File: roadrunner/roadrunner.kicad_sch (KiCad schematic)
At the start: 48 parts, among them J1 Battery_conn, J2 battery_conn_r, SW1 SW_Push, SW10 SW_Push, SW10_r1 SW_Push, SW11 SW_Push, SW11_r1 SW_Push, SW12 SW_Push, SW12_r1 SW_Push, SW13 SW_Push, SW13_r1 SW_Push, SW14 SW_Push, SW14_r1 SW_Push, SW15 SW_Push, SW15_r1 SW_Push, SW16 SW_Push, SW16_r1 SW_Push, SW17 SW_Push, SW17_r1 SW_Push, SW1_r1 SW_Push, SW2 SW_Push, SW2_r1 SW_Push, SW3 SW_Push, SW3_r1 SW_Push, SW4 SW_Push, SW4_r1 SW_Push, SW5 SW_Push, SW5_r1 SW_Push, SW6 SW_Push, SW6_r1 SW_Push, SW7 SW_Push, SW7_r1 SW_Push, SW8 SW_Push, SW8_r1 SW_Push, SW9 SW_Push, SW9_r1 SW_Push, U1 ProMicro-kbd, U2 ProMicro-kbd

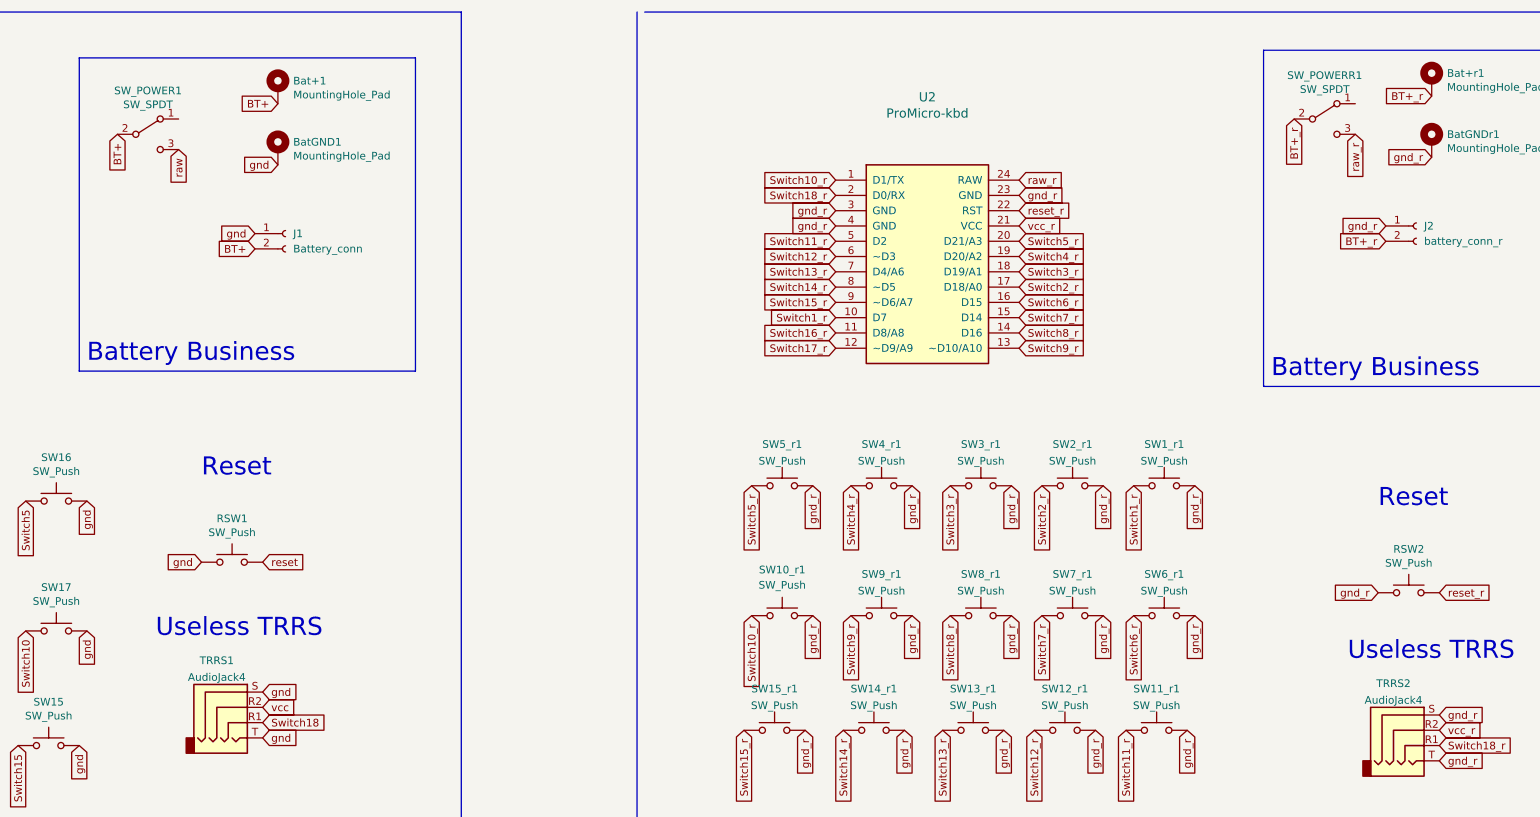
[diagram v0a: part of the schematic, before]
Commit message: update shape
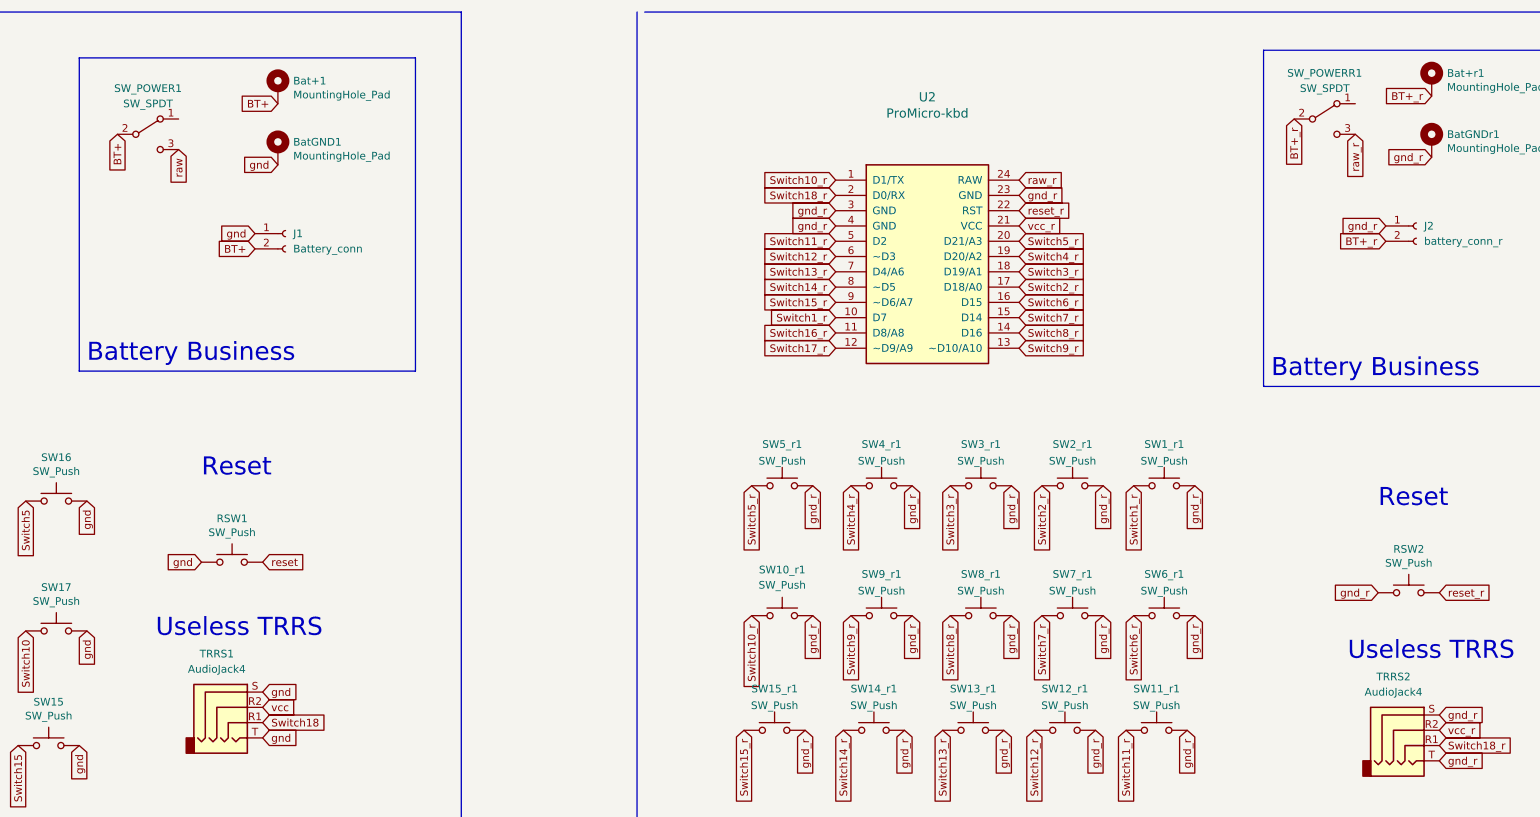
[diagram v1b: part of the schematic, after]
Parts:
- TRRS1, TRRS2: footprint (none) -> Connector_Audio:Jack_3.5mm_PJ320E_Horizontal
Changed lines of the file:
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@@
   (symbol (lib_id "Connector:AudioJack4") (at 331.47 133.35 0) (unit 1)
     (in_bom yes) (on_board yes) (fields_autoplaced)
-    (property "Reference" "TRRS2" (id 0) (at 328.93 125.5735 0))
-    (property "Value" "AudioJack4" (id 1) (at 328.93 128.3486 0))
-    (property "Footprint" "" (id 2) (at 331.47 133.35 0)
+    (property "Reference" "TRRS2" (id 0) (at 328.93 124.46 0))
+    (property "Value" "AudioJack4" (id 1) (at 328.93 127 0))
+    (property "Footprint" "Connector_Audio:Jack_3.5mm_PJ320E_Horizontal" (id 2) (at 331.47 133.35 0)
       (effects (font (size 1.27 1.27)) hide)
     )
@@
   (symbol (lib_id "Connector:AudioJack4") (at 135.89 129.54 0) (unit 1)
     (in_bom yes) (on_board yes) (fields_autoplaced)
-    (property "Reference" "TRRS1" (id 0) (at 133.35 121.7635 0))
-    (property "Value" "AudioJack4" (id 1) (at 133.35 124.5386 0))
-    (property "Footprint" "" (id 2) (at 135.89 129.54 0)
+    (property "Reference" "TRRS1" (id 0) (at 133.35 120.65 0))
+    (property "Value" "AudioJack4" (id 1) (at 133.35 123.19 0))
+    (property "Footprint" "Connector_Audio:Jack_3.5mm_PJ320E_Horizontal" (id 2) (at 135.89 129.54 0)
       (effects (font (size 1.27 1.27)) hide)
     )
@@
   )
   (symbol (lib_id "Switch:SW_SPDT") (at 121.92 34.29 0) (unit 1)
-    (in_bom yes) (on_board yes)
-    (property "Reference" "SW_POWER1" (id 0) (at 121.92 27.051 0))
-    (property "Value" "SW_SPDT" (id 1) (at 121.92 29.3624 0))
+    (in_bom yes) (on_board yes) (fields_autoplaced)
+    (property "Reference" "SW_POWER1" (id 0) (at 121.92 26.67 0))
+    (property "Value" "SW_SPDT" (id 1) (at 121.92 29.21 0))
     (property "Footprint" "battery_switch:SPDT_C128955" (id 2) (at 121.92 34.29 0)
       (effects (font (size 1.27 1.27)) hide)
@@
   )
   (symbol (lib_id "Switch:SW_SPDT") (at 317.5 31.75 0) (unit 1)
-    (in_bom yes) (on_board yes)
-    (property "Reference" "SW_POWERR1" (id 0) (at 317.5 24.511 0))
-    (property "Value" "SW_SPDT" (id 1) (at 317.5 26.8224 0))
+    (in_bom yes) (on_board yes) (fields_autoplaced)
+    (property "Reference" "SW_POWERR1" (id 0) (at 317.5 24.13 0))
+    (property "Value" "SW_SPDT" (id 1) (at 317.5 26.67 0))
     (property "Footprint" "battery_switch:SPDT_C128955" (id 2) (at 317.5 31.75 0)
       (effects (font (size 1.27 1.27)) hide)
@@
     )
     (path "/5707fb00-48c3-46d9-8f62-42ff2e9ad9f5"
-      (reference "TRRS1") (unit 1) (value "AudioJack4") (footprint "")
+      (reference "TRRS1") (unit 1) (value "AudioJack4") (footprint "Connector_Audio:Jack_3.5mm_PJ320E_Horizontal")
     )
     (path "/5340d998-a6ef-44fa-806e-718c814691ee"
-      (reference "TRRS2") (unit 1) (value "AudioJack4") (footprint "")
+      (reference "TRRS2") (unit 1) (value "AudioJack4") (footprint "Connector_Audio:Jack_3.5mm_PJ320E_Horizontal")
     )
     (path "/6801880a-11a2-4a6a-9688-e81ed1f59985"

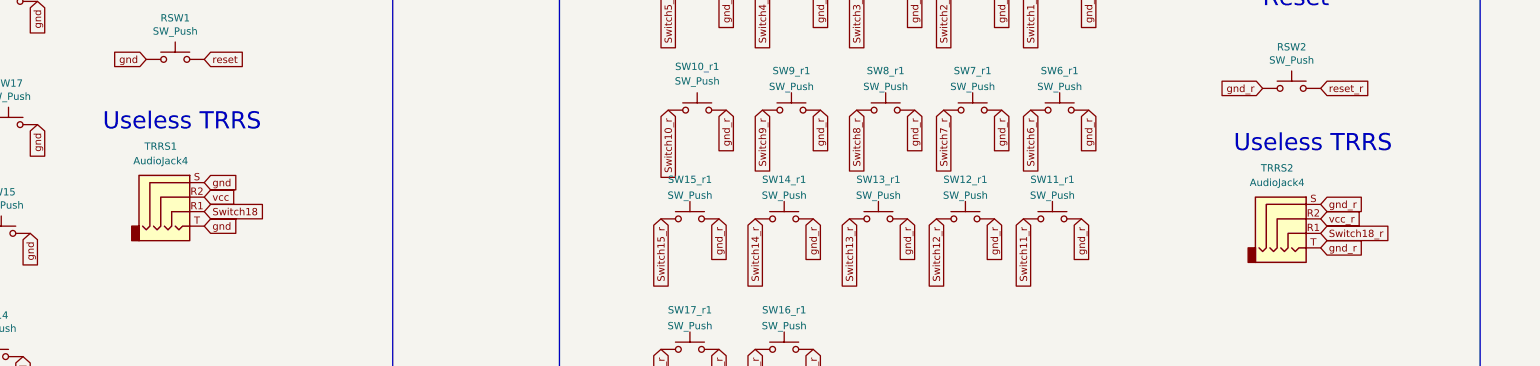
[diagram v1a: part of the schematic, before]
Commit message: basic v2 designs
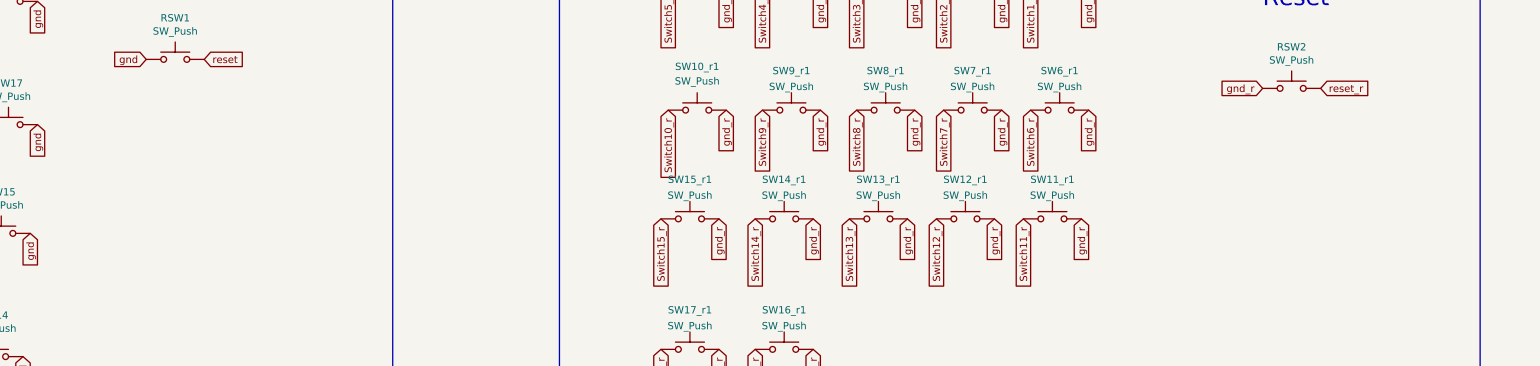
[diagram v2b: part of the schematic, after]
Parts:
- removed TRRS1, TRRS2: AudioJack4, Connector_Audio:Jack_3.5mm_PJ320E_Horizontal, symbol Connector:AudioJack4
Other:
- note removed: "Useless TRRS"
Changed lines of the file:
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@@
-    (effects (font (size 2.9972 2.9972)) (justify left bottom))
-  )
-  (text "Useless TRRS\n" (at 321.31 121.92 0)
     (effects (font (size 2.9972 2.9972)) (justify left bottom))
   )
@@
     (effects (font (size 2.9972 2.9972)) (justify left bottom))
   )
-  (text "Useless TRRS\n" (at 123.19 118.11 0)
-    (effects (font (size 2.9972 2.9972)) (justify left bottom))
-  )
   (text "Battery Business" (at 308.61 74.93 0)
     (effects (font (size 2.9972 2.9972)) (justify left bottom))
@@
     )
   )
-  (global_label "vcc_r" (shape input) (at 336.55 133.35 0) (fields_autoplaced)
-    (effects (font (size 1.27 1.27)) (justify left))
-    (property "Intersheet References" "${INTERSHEET_REFS}" (id 0) (at 343.7728 133.2706 0)
-      (effects (font (size 1.27 1.27)) (justify left) hide)
-    )
-  )
   (global_label "gnd" (shape input) (at 80.01 95.25 270) (fields_autoplaced)
     (effects (font (size 1.27 1.27)) (justify right))
     (property "Intersheet References" "${INTERSHEET_REFS}" (id 0) (at 13.97 66.04 0)
-      (effects (font (size 1.27 1.27)) hide)
-    )
-  )
-  (global_label "gnd" (shape input) (at 140.97 134.62 0) (fields_autoplaced)
-    (effects (font (size 1.27 1.27)) (justify left))
-    (property "Intersheet References" "${INTERSHEET_REFS}" (id 0) (at 13.97 67.31 0)
       (effects (font (size 1.27 1.27)) hide)
     )
@@
     )
   )
-  (global_label "gnd" (shape input) (at 140.97 127 0) (fields_autoplaced)
-    (effects (font (size 1.27 1.27)) (justify left))
-    (property "Intersheet References" "${INTERSHEET_REFS}" (id 0) (at 13.97 59.69 0)
-      (effects (font (size 1.27 1.27)) hide)
-    )
-  )
   (global_label "Switch5" (shape input) (at 101.6 95.25 270) (fields_autoplaced)
     (effects (font (size 1.27 1.27)) (justify right))
@@
     (property "Intersheet References" "${INTERSHEET_REFS}" (id 0) (at 13.97 66.04 0)
       (effects (font (size 1.27 1.27)) hide)
-    )
-  )
-  (global_label "gnd_r" (shape input) (at 336.55 130.81 0) (fields_autoplaced)
-    (effects (font (size 1.27 1.27)) (justify left))
-    (property "Intersheet References" "${INTERSHEET_REFS}" (id 0) (at 344.0752 130.8894 0)
-      (effects (font (size 1.27 1.27)) (justify left) hide)
     )
   )
@@
     )
   )
-  (global_label "gnd_r" (shape input) (at 336.55 138.43 0) (fields_autoplaced)
-    (effects (font (size 1.27 1.27)) (justify left))
-    (property "Intersheet References" "${INTERSHEET_REFS}" (id 0) (at 344.0752 138.5094 0)
-      (effects (font (size 1.27 1.27)) (justify left) hide)
-    )
-  )
   (global_label "raw" (shape input) (at 127 36.83 270) (fields_autoplaced)
     (effects (font (size 1.27 1.27)) (justify right))
@@
     )
   )
-  (global_label "Switch18" (shape input) (at 140.97 132.08 0) (fields_autoplaced)
-    (effects (font (size 1.27 1.27)) (justify left))
-    (property "Intersheet References" "${INTERSHEET_REFS}" (id 0) (at 13.97 67.31 0)
-      (effects (font (size 1.27 1.27)) hide)
-    )
-  )
   (global_label "reset_r" (shape input) (at 336.55 110.49 0) (fields_autoplaced)
     (effects (font (size 1.27 1.27)) (justify left))
@@
     )
   )
-  (global_label "vcc" (shape input) (at 140.97 129.54 0) (fields_autoplaced)
-    (effects (font (size 1.27 1.27)) (justify left))
-    (property "Intersheet References" "${INTERSHEET_REFS}" (id 0) (at 13.97 59.69 0)
-      (effects (font (size 1.27 1.27)) hide)
-    )
-  )
   (global_label "gnd_r" (shape input) (at 265.43 92.71 270) (fields_autoplaced)
     (effects (font (size 1.27 1.27)) (justify right))
@@
     (property "Intersheet References" "${INTERSHEET_REFS}" (id 0) (at 285.6706 104.1056 90)
       (effects (font (size 1.27 1.27)) (justify right) hide)
-    )
-  )
-  (global_label "Switch18_r" (shape input) (at 336.55 135.89 0) (fields_autoplaced)
-    (effects (font (size 1.27 1.27)) (justify left))
-    (property "Intersheet References" "${INTERSHEET_REFS}" (id 0) (at 208.28 -27.94 0)
-      (effects (font (size 1.27 1.27)) hide)
     )
   )
@@
     (pin "2")
   )
-  (symbol (lib_id "Connector:AudioJack4") (at 331.47 133.35 0) (unit 1)
-    (in_bom yes) (on_board yes) (fields_autoplaced)
-    (property "Reference" "TRRS2" (id 0) (at 328.93 124.46 0))
-    (property "Value" "AudioJack4" (id 1) (at 328.93 127 0))
-    (property "Footprint" "Connector_Audio:Jack_3.5mm_PJ320E_Horizontal" (id 2) (at 331.47 133.35 0)
-      (effects (font (size 1.27 1.27)) hide)
-    )
-    (property "Datasheet" "~" (id 3) (at 331.47 133.35 0)
-      (effects (font (size 1.27 1.27)) hide)
-    )
-    (pin "R1")
-    (pin "R2")
-    (pin "S")
-    (pin "T")
-  )
-  (symbol (lib_id "Connector:AudioJack4") (at 135.89 129.54 0) (unit 1)
-    (in_bom yes) (on_board yes) (fields_autoplaced)
-    (property "Reference" "TRRS1" (id 0) (at 133.35 120.65 0))
-    (property "Value" "AudioJack4" (id 1) (at 133.35 123.19 0))
-    (property "Footprint" "Connector_Audio:Jack_3.5mm_PJ320E_Horizontal" (id 2) (at 135.89 129.54 0)
-      (effects (font (size 1.27 1.27)) hide)
-    )
-    (property "Datasheet" "~" (id 3) (at 135.89 129.54 0)
-      (effects (font (size 1.27 1.27)) hide)
-    )
-    (pin "R1")
-    (pin "R2")
-    (pin "S")
-    (pin "T")
-  )
   (symbol (lib_id "Connector:Conn_01x02_Female") (at 332.74 49.53 0) (unit 1)
     (in_bom yes) (on_board yes) (fields_autoplaced)
@@
       (reference "SW_POWERR1") (unit 1) (value "SW_SPDT") (footprint "battery_switch:SPDT_C128955")
     )
-    (path "/5707fb00-48c3-46d9-8f62-42ff2e9ad9f5"
-      (reference "TRRS1") (unit 1) (value "AudioJack4") (footprint "Connector_Audio:Jack_3.5mm_PJ320E_Horizontal")
-    )
-    (path "/5340d998-a6ef-44fa-806e-718c814691ee"
-      (reference "TRRS2") (unit 1) (value "AudioJack4") (footprint "Connector_Audio:Jack_3.5mm_PJ320E_Horizontal")
-    )
     (path "/6801880a-11a2-4a6a-9688-e81ed1f59985"
